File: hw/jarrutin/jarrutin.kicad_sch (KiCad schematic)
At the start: 27 parts, among them Q1 TCRT5000L, Q2 IRFIZ34NPdF, SW1 RESET, U1 40106, U2 TC4420, U3 L7805, U4 Pico

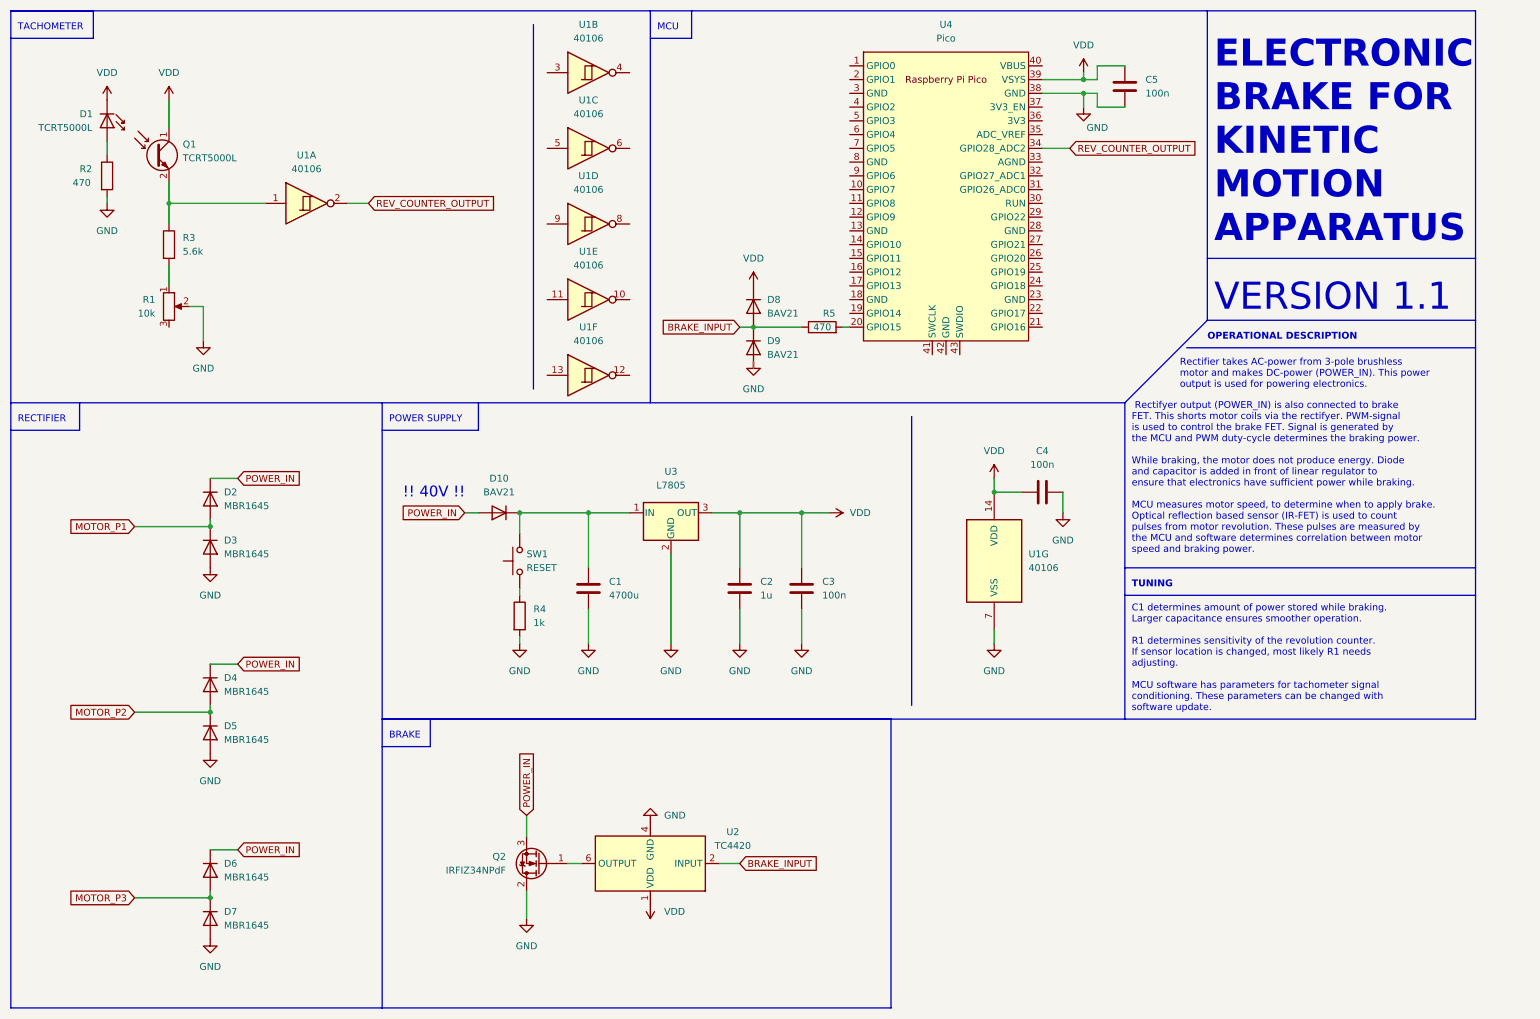
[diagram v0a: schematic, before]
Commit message: Updated schematic
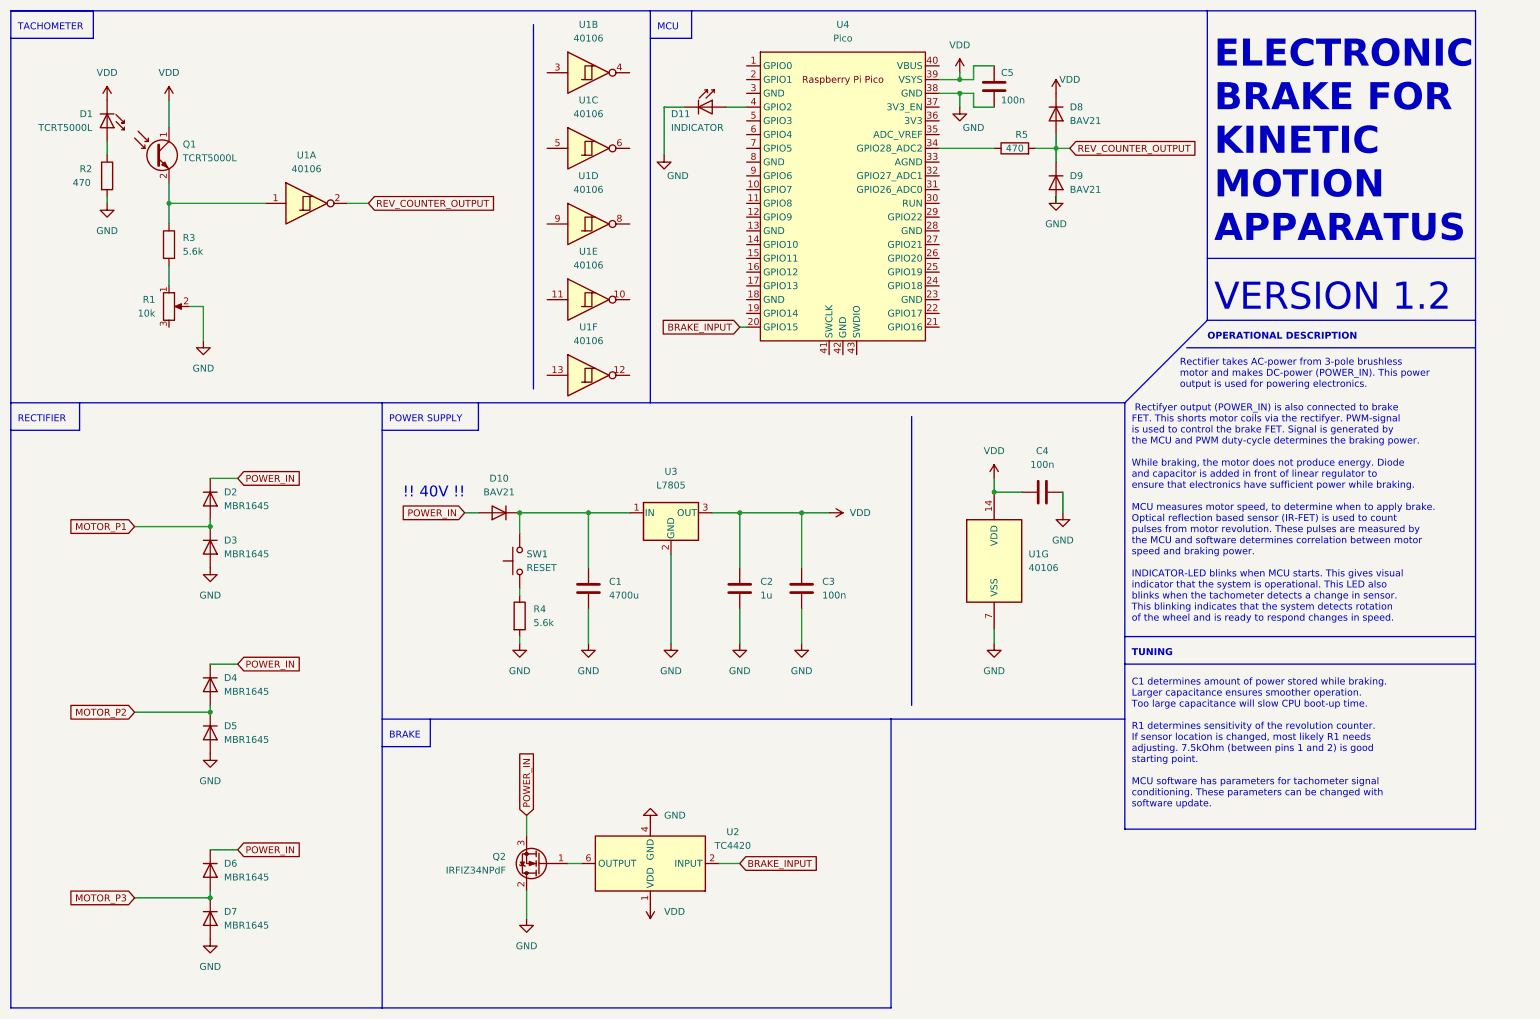
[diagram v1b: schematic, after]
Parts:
- added D11: INDICATOR, symbol LED:IR204A
- R4: value 1k -> 5.6k
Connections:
- net BRAKE_INPUT: now also U4.20 (GPIO15); no longer D8.2 (A), D9.1 (K), R5.1
- net GND: now also D11.1 (K)
- net REV_COUNTER_OUTPUT: now also D8.2 (A), D9.1 (K), R5.2; no longer U4.34 (GPIO28_ADC2)
- net at U4.4 (GPIO2): now also D11.2 (A)
- new net: R5.1, U4.34 (GPIO28_ADC2)
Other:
- note added: "C1 determines amount of power stored while braking. Larger capacitance ensures smoother operation. Too large capacitance will slow CPU boot-up time. R1 determines sensitivity of the revolution counter. If sensor location is changed, most likely R1 needs adjusting. 7.5kOhm (between pins 1 and 2) is good starting point. MCU software has parameters for tachometer signal conditioning. These parameter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"
- note added: "VERSION 1.2"
- note removed: "C1 determines amount of power stored while braking. Larger capacitance ensures smoother operation. R1 determines sensitivity of the revolution counter. If sensor location is changed, most likely R1 needs adjusting. MCU software has parameters for tachometer signal conditioning. These parameters can be changed with software update."
- note removed: "VERSION 1.1"
- moved on the sheet: C5, D8, D9, R5, U4
